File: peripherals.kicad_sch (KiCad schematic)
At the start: 36 parts, among them J5 DB25_Male, J6 Conn_02x08_Odd_Even, Q25 BC856B, U16 ISL83485IBZ, U25 BSP16T1G, U29 LM358

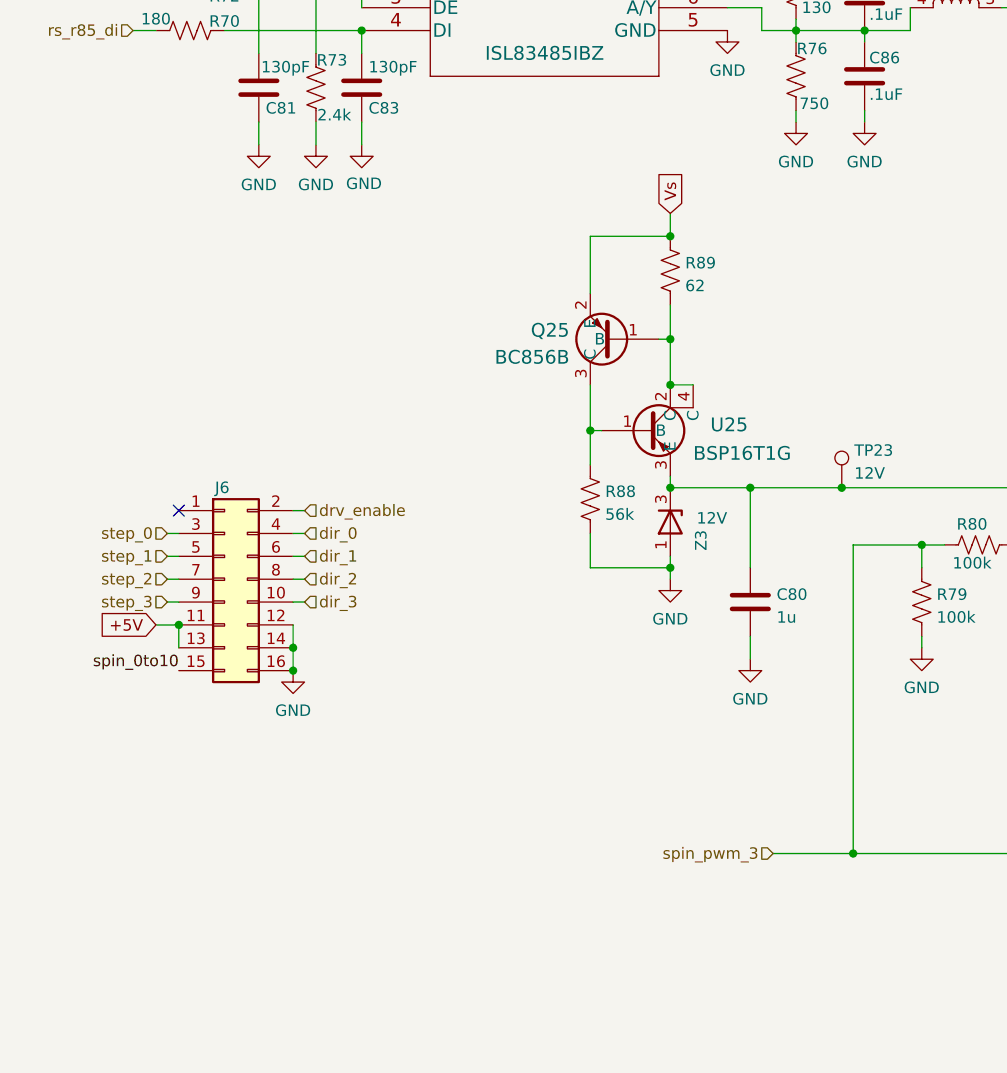
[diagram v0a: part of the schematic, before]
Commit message: changed 12V supply for 0-10V out to LDO voltage regulator
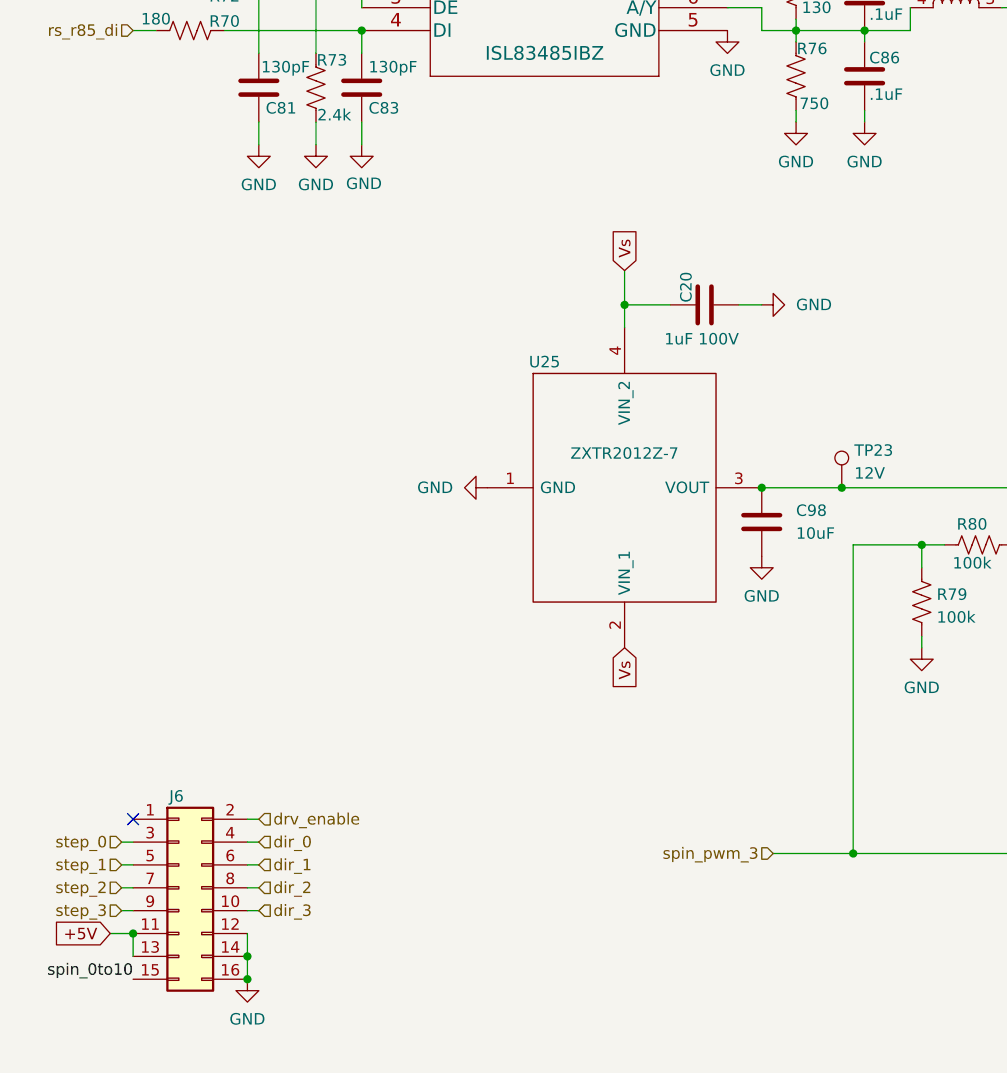
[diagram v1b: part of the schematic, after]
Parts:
- removed C80: 1u, Capacitor_SMD:C_0805_2012Metric_Pad1.18x1.45mm_HandSolder, symbol Device:C
- removed Q25: BC856B, Project_Footprints_Library:BC856B_215, symbol 1LibBBCTRL:BC856B
- removed R88: 56k, Resistor_SMD:R_0805_2012Metric_Pad1.20x1.40mm_HandSolder, symbol Device:R_US
- removed R89: 62, Resistor_SMD:R_0805_2012Metric_Pad1.20x1.40mm_HandSolder, symbol Device:R_US
- removed U25: BSP16T1G, Project_Footprints_Library:BSP16T1G, symbol 1LibBBCTRL:BSP16T1G
- removed Z3: 12V, Package_TO_SOT_SMD:SOT-23, symbol 1LibBBCTRL:MMBZ5242BLT3G
- added C20: 1uF 100V, Capacitor_SMD:C_0805_2012Metric_Pad1.18x1.45mm_HandSolder, symbol Device:C
- added C98: 10uF, Capacitor_SMD:C_1206_3216Metric_Pad1.33x1.80mm_HandSolder, symbol Device:C
- added U25: ZXTR2012Z-7, Project_Footprints_Library:ZXTR2012Z7, symbol 1LibBBCTRL:ZXTR2012Z-7
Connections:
- net GND: now also C20.2, C98.2, U25.1 (GND)
- net Vs: now also C20.1, U25.2 (VIN_1), U25.4 (VIN_2)
- net at C96.1, TP23.1, U29.8 (V+): now also C98.1, U25.3 (VOUT)
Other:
- moved on the sheet: J6
